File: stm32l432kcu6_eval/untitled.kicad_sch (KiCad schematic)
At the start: 7 parts, among them J3 USB_C_Receptacle, U2 XC6206PxxxMR, U3 USBLC6-2SC6

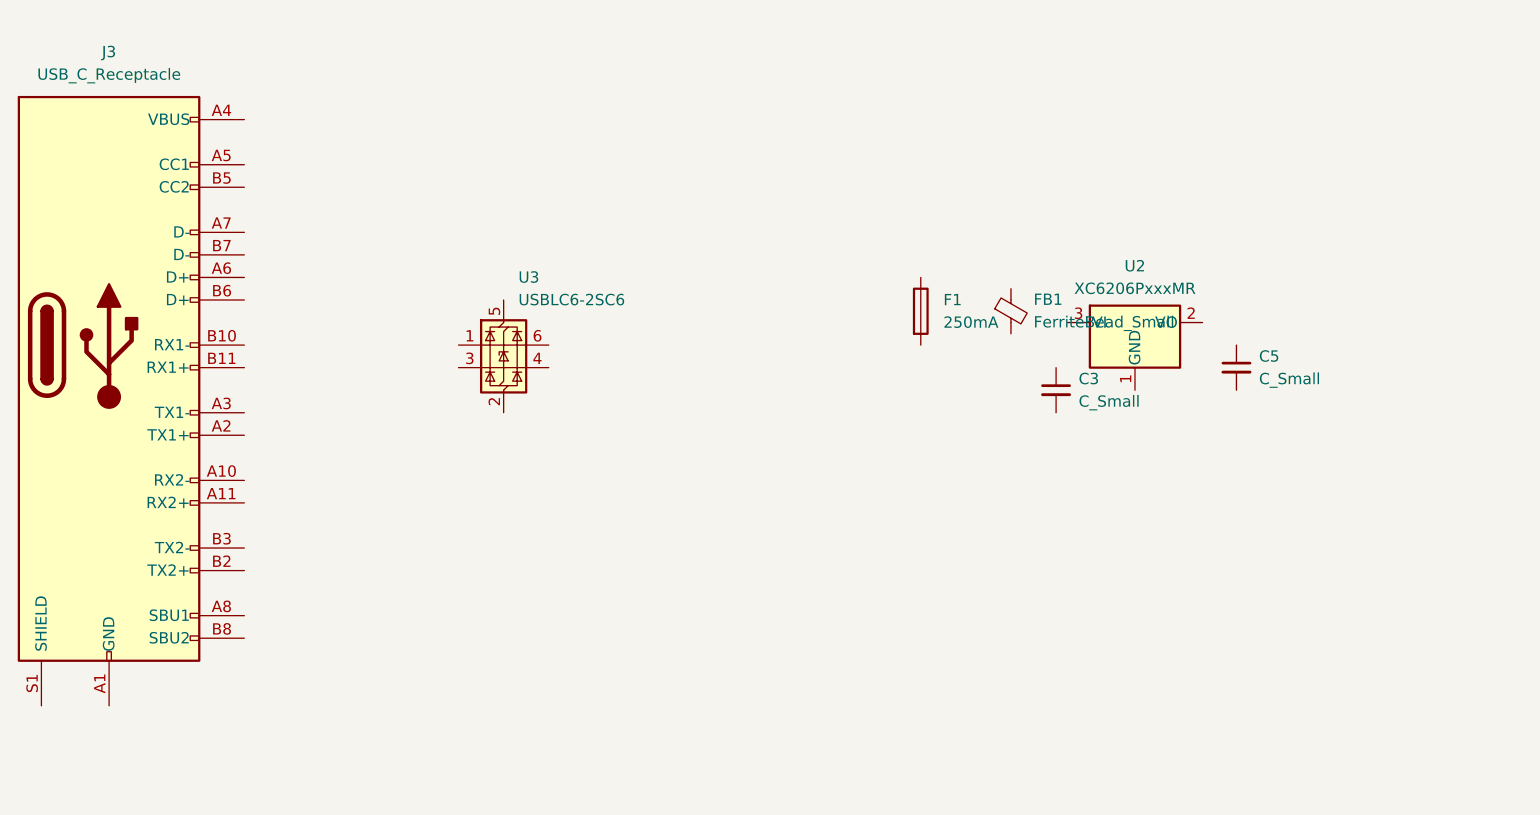
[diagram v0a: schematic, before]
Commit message: board save 1
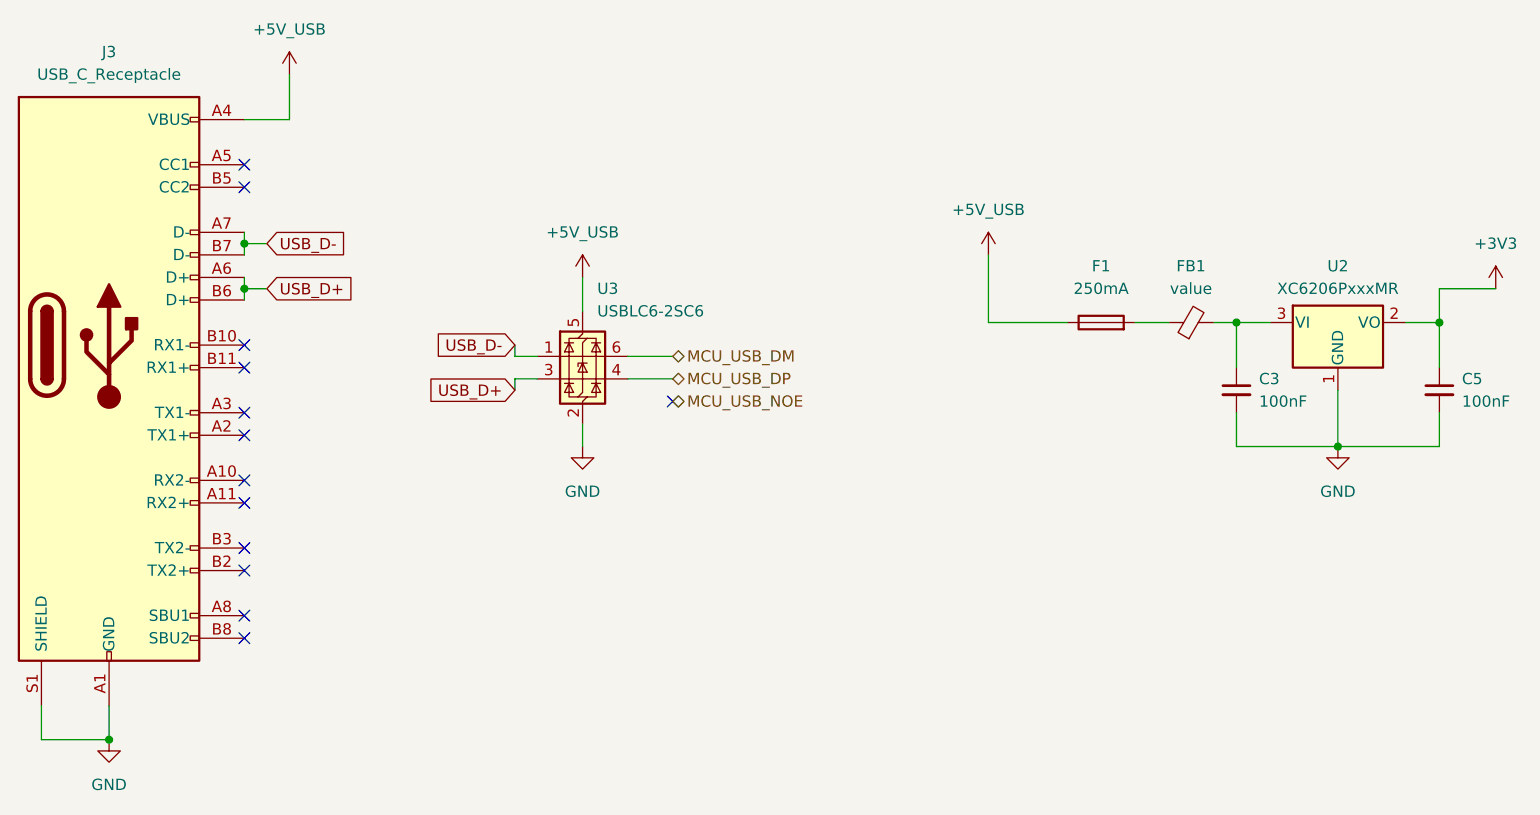
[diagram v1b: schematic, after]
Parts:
- C3, C5: value C_Small -> 100nF
- FB1: value FerriteBead_Small -> value
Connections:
- net +5V_USB: now reaches F1.1
- net +5V_USB: now also J3.A4 (VBUS), J3.A9 (VBUS), J3.B4 (VBUS), J3.B9 (VBUS), U3.5 (VBUS)
- net at F1.2: now also FB1.1
- net +3V3: now reaches C5.1
- net +3V3: now also U2.2 (VO)
- net GND: now reaches C5.2
- net GND: now also C3.2, J3.A1 (GND), J3.A12 (GND), J3.B1 (GND), J3.B12 (GND), J3.S1 (SHIELD), U2.1 (GND), U3.2 (GND)
- net at U2.3 (VI): now also C3.1, FB1.2
- net USB_D-: now reaches U3.1 (I/O1)
- net USB_D-: now also J3.A7 (D-), J3.B7 (D-)
- net USB_D+: now reaches U3.3 (I/O2)
- net USB_D+: now also J3.A6 (D+), J3.B6 (D+)
- net MCU_USB_DP: now reaches U3.4 (I/O2)
- net MCU_USB_DM: now reaches U3.6 (I/O1)
- no-connect marks 0 -> 13
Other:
- moved on the sheet: C3, C5, F1, FB1, U2, U3
